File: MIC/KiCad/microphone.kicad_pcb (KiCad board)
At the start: 2 copper layers, 43.5 x 34 mm, 17 parts, among them J1 Conn_01x06_Pin, U1 LMV321

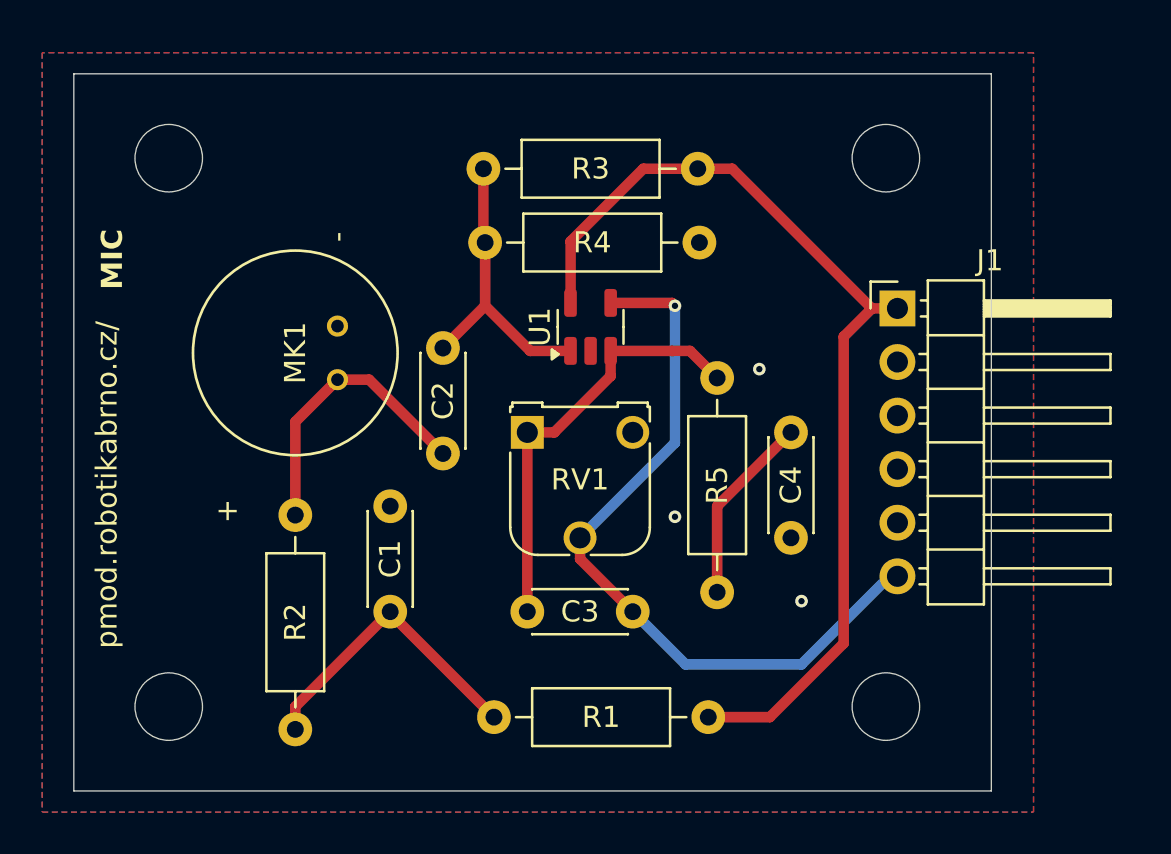
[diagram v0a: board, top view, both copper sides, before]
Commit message: Deployed d972a79 with MkDocs version: 1.6.0
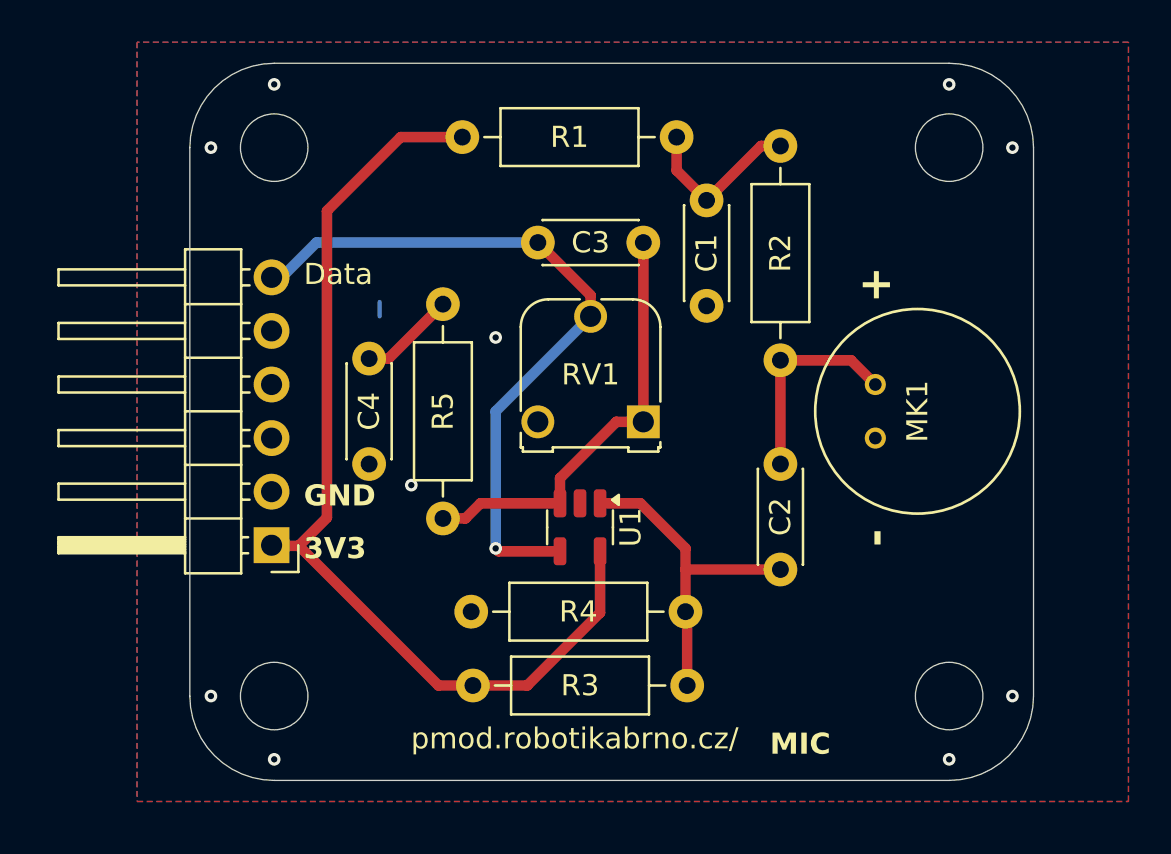
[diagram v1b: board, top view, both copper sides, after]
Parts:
- moved H3 45.5 mm to (144.0, 87.5), turned to 180 degrees
- moved H2 44.9 mm to (144.0, 113.5), turned to 180 degrees
- moved H4 39.3 mm to (112.0, 87.5), turned to 180 degrees
- moved H1 38.6 mm to (112.0, 113.5), turned to 180 degrees
- moved R2 36.0 mm to (136.0, 87.4), turned to -90 degrees
- moved J1 31.7 mm to (111.9, 106.3), turned to 180 degrees
- moved MK1 29.6 mm to (142.5, 100.0), turned to -90 degrees
- moved R1 28.8 mm to (131.1, 87.0), turned to 180 degrees
- moved R3 26.7 mm to (121.4, 113.0), turned to 0 degrees
- moved C1 24.6 mm to (132.5, 90.0), turned to -90 degrees
- moved C4 20.3 mm to (116.5, 97.5)
- moved R4 19.9 mm to (131.5, 109.5), turned to 180 degrees
- moved R5 18.9 mm to (120.0, 94.9), turned to -90 degrees
- moved C3 18.1 mm to (124.5, 92.0), turned to 0 degrees
- moved C2 16.0 mm to (136.0, 102.5), turned to -90 degrees
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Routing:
- net Net-(C1-Pad1): track 14.5 -> 8.16 mm
- net Net-(C4-Pad1): track 9.03 -> 4.57 mm
- net Net-(C2-Pad1): track 13.7 -> 9.90 mm
- net Net-(J1-Pin_6): track 35.8 -> 33.7 mm
- net Net-(U1-+): track 14.3 -> 16.0 mm
- net GND: vias 3 -> 10
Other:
- board size 43.5 x 34 mm -> 40 x 34 mm
- board text added: "3V3"
- board text added: "Data"
- board text added: "GND"
